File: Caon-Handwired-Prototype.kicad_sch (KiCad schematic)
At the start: 11 parts, among them U1 74HC595, U2 SuperMini nRF52840

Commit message: Schematic Update
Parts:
- S_C1: footprint Caon65:Capacitor_0805 -> Caon_Footprint:Capacitor_0805
- S_D1, S_D2, S_D3, S_D4, S_D5, S_D6, S_D7, S_D8: footprint Caon65:D_SOD-123_1N4148W -> Caon_Footprint:D_SOD-123_1N4148W
- U1: footprint Caon65:74HC595A -> Caon_Footprint:74HC595A
- U2: footprint PCM_marbastlib-xp-promicroish:SuperMini_nRF52840_AH_USBup -> Caon_Footprint:SuperMini_NiceNano_USBdn
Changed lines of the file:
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@@
 			)
 		)
-		(property "Footprint" "Caon65:D_SOD-123_1N4148W"
+		(property "Footprint" "Caon_Footprint:D_SOD-123_1N4148W"
 			(at 152.4 48.26 0)
 			(effects
@@
 			)
 		)
-		(property "Footprint" "Caon65:D_SOD-123_1N4148W"
+		(property "Footprint" "Caon_Footprint:D_SOD-123_1N4148W"
 			(at 152.4 38.1 0)
 			(effects
@@
 			)
 		)
-		(property "Footprint" "Caon65:D_SOD-123_1N4148W"
+		(property "Footprint" "Caon_Footprint:D_SOD-123_1N4148W"
 			(at 152.4 43.18 0)
 			(effects
@@
 			)
 		)
-		(property "Footprint" "Caon65:D_SOD-123_1N4148W"
+		(property "Footprint" "Caon_Footprint:D_SOD-123_1N4148W"
 			(at 152.4 53.34 0)
 			(effects
@@
 			)
 		)
-		(property "Footprint" "Caon65:74HC595A"
+		(property "Footprint" "Caon_Footprint:74HC595A"
 			(at 129.54 48.26 0)
 			(effects
@@
 			)
 		)
-		(property "Footprint" "Caon65:D_SOD-123_1N4148W"
+		(property "Footprint" "Caon_Footprint:D_SOD-123_1N4148W"
 			(at 143.51 50.8 0)
 			(effects
@@
 			)
 		)
-		(property "Footprint" "Caon65:D_SOD-123_1N4148W"
+		(property "Footprint" "Caon_Footprint:D_SOD-123_1N4148W"
 			(at 143.51 55.88 0)
 			(effects
@@
 			)
 		)
-		(property "Footprint" "Caon65:Capacitor_0805"
+		(property "Footprint" "Caon_Footprint:Capacitor_0805"
 			(at 110.49 49.53 0)
 			(effects
@@
 			)
 		)
-		(property "Footprint" "Caon65:D_SOD-123_1N4148W"
+		(property "Footprint" "Caon_Footprint:D_SOD-123_1N4148W"
 			(at 143.51 40.64 0)
 			(effects
@@
 			)
 		)
-		(property "Footprint" "Caon65:D_SOD-123_1N4148W"
+		(property "Footprint" "Caon_Footprint:D_SOD-123_1N4148W"
 			(at 143.51 45.72 0)
 			(effects
@@
 			)
 		)
-		(property "Footprint" "PCM_marbastlib-xp-promicroish:SuperMini_nRF52840_AH_USBup"
+		(property "Footprint" "Caon_Footprint:SuperMini_NiceNano_USBdn"
 			(at 63.5 81.28 0)
 			(effects

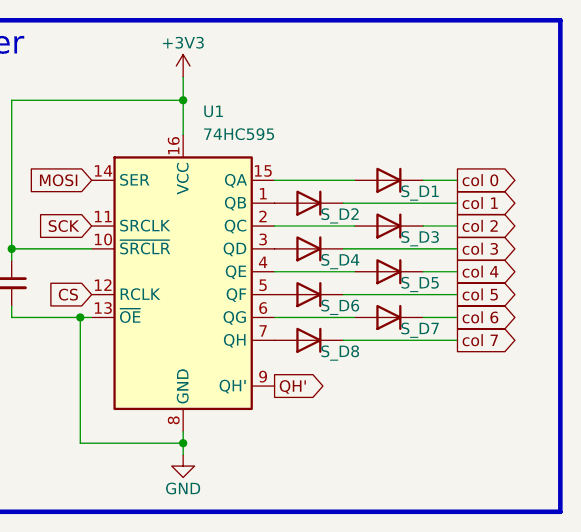
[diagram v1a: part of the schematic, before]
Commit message: Schematic update
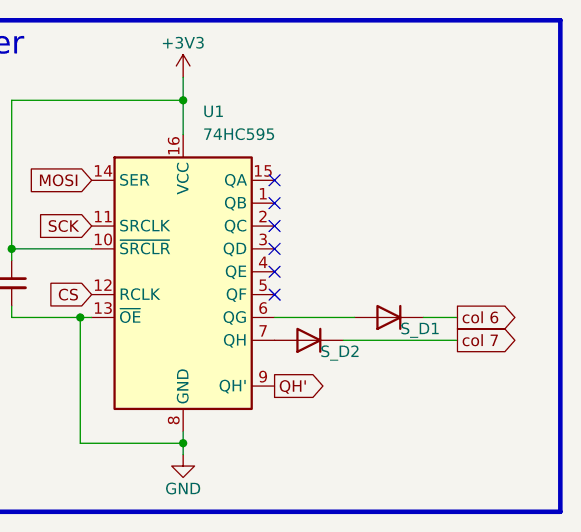
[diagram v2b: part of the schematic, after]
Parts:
- removed S_D1, S_D2, S_D3, S_D4, S_D5, S_D6: 1N4148, Caon_Footprint:D_SOD-123_1N4148W, symbol Caon65:Diode_1N4148W_SOD-123
- renumbered S_D7 to S_D1, S_D8 to S_D2
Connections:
- no-connect marks 15 -> 21
